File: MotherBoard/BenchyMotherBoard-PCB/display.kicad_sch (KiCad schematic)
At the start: 13 parts

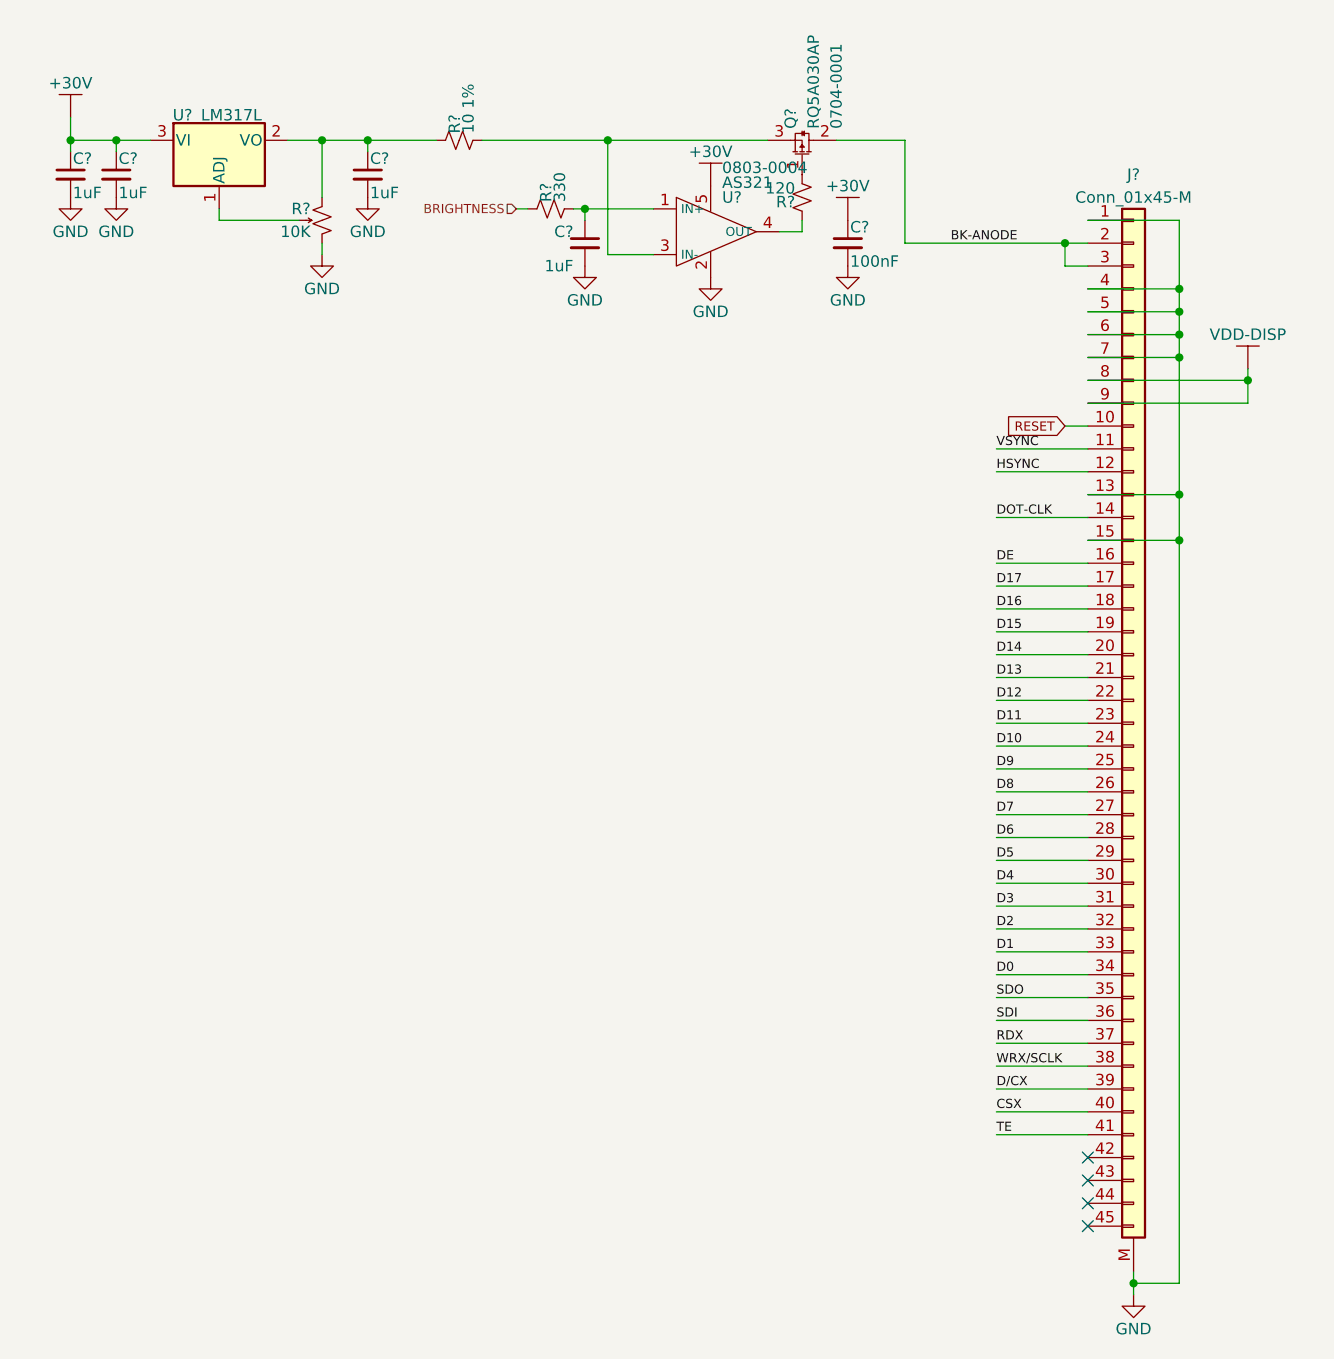
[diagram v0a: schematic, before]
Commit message: Initial schematic lock
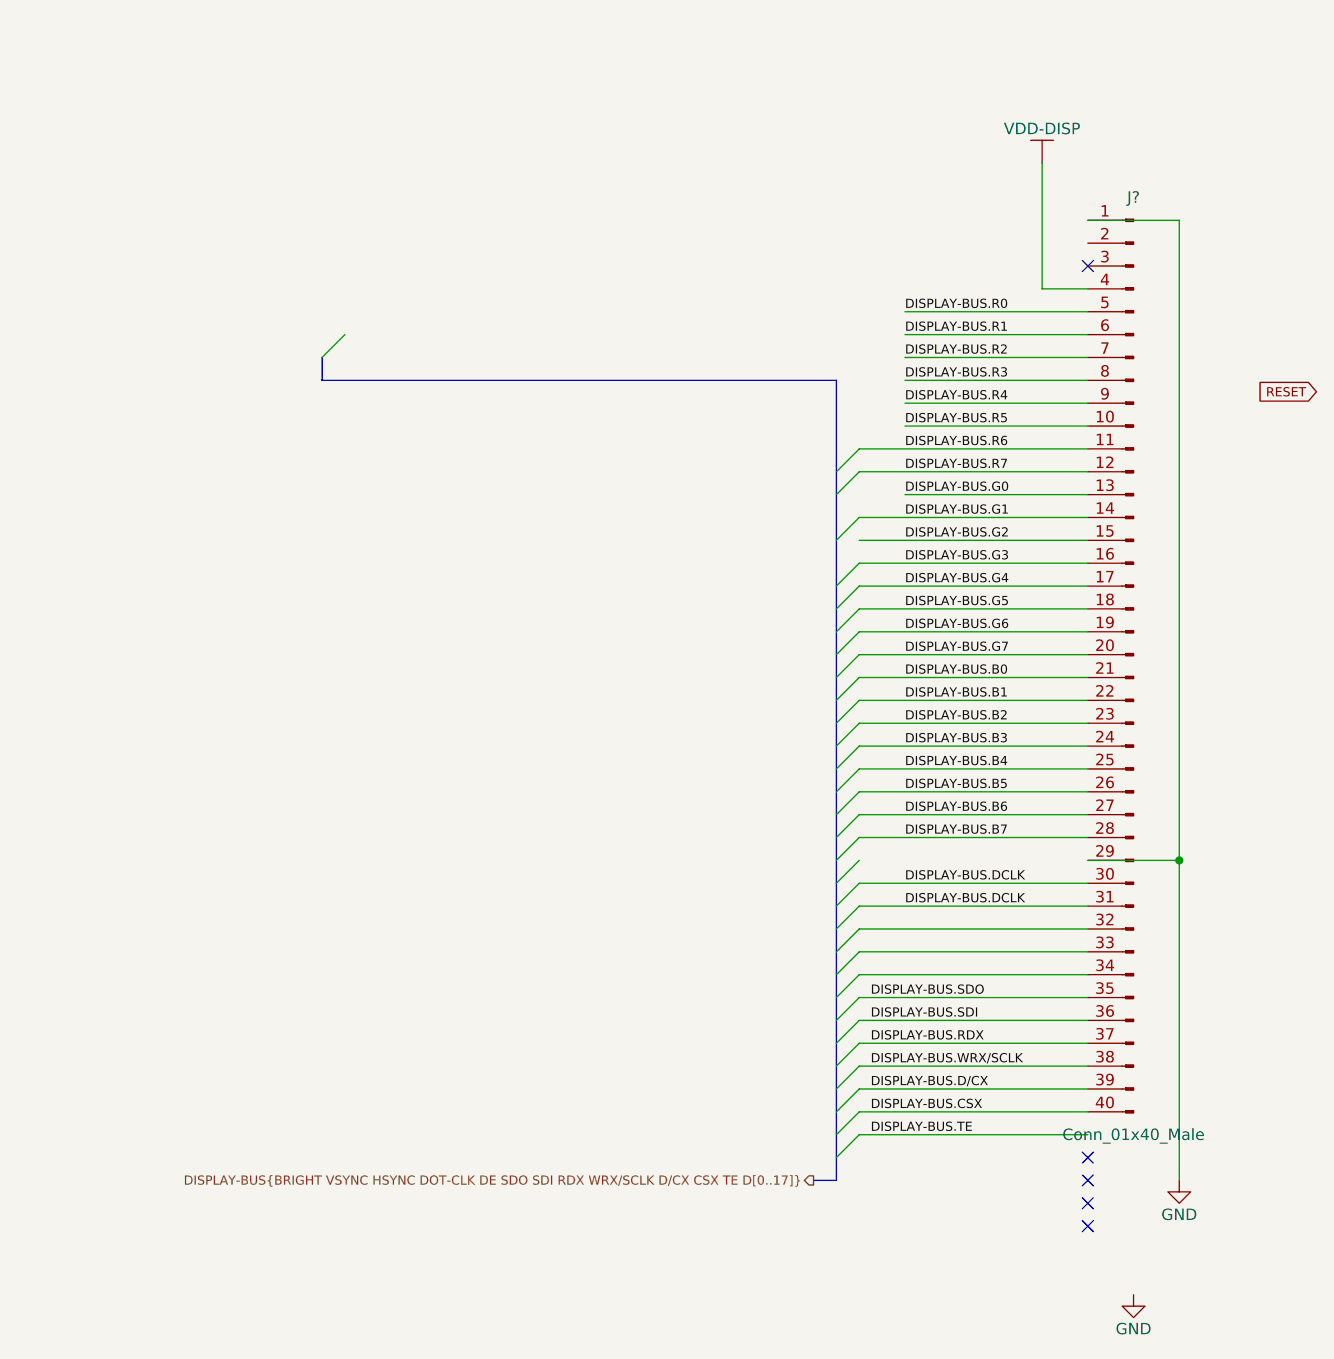
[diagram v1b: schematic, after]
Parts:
- removed C?: 1uF, symbol Device:C_Small
- removed C?: 1uF, Capacitor_SMD:C_0805_2012Metric, symbol Device:C_Small
- removed C? (x2): 1uF, Capacitor_SMD:C_1210_3225Metric, symbol Device:C_Small
- removed C?: 100nF, Capacitor_SMD:C_0805_2012Metric, symbol Device:C_Small
- removed J?: Conn_01x45-M, Daxxn_Connectors:046841045100846+, symbol Daxxn_Connectors:Conn_01x45-M
- removed Q?: RQ5A030AP, Package_TO_SOT_SMD:SOT-23, symbol Daxxn_Transistors:RQ5A030AP
- removed R?: 120, Resistor_SMD:R_0805_2012Metric, symbol Device:R_Small_US
- removed R?: 10K, symbol Daxxn_Other:R_Pot_Small_US
- removed R?: 330, Resistor_SMD:R_0805_2012Metric, symbol Device:R_Small_US
- removed R?: 10 1%, Resistor_SMD:R_0805_2012Metric, symbol Device:R_Small_US
- removed U?: AS321, Package_TO_SOT_SMD:SOT-23-5, symbol Daxxn_OPAMP:AS321
- removed U?: LM317L, Package_TO_SOT_SMD:SOT-89-3, symbol Regulator_Linear:LM317L_SOT-89
- added J?: Conn_01x40_Male, symbol Connector:Conn_01x40_Male
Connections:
- net GND: now also J?.1 (Pin_1), J?.29 (Pin_29)
- net VDD-DISP: now also J?.4 (Pin_4)
- new net DISPLAY-BUS.B0: J?.21 (Pin_21)
- new net DISPLAY-BUS.B1: J?.22 (Pin_22)
- new net DISPLAY-BUS.B2: J?.23 (Pin_23)
- new net DISPLAY-BUS.B3: J?.24 (Pin_24)
- new net DISPLAY-BUS.B4: J?.25 (Pin_25)
- new net DISPLAY-BUS.B5: J?.26 (Pin_26)
- new net DISPLAY-BUS.B6: J?.27 (Pin_27)
- new net DISPLAY-BUS.B7: J?.28 (Pin_28)
- new net DISPLAY-BUS.CSX: J?.40 (Pin_40)
- new net DISPLAY-BUS.DCLK: J?.30 (Pin_30), J?.31 (Pin_31)
- new net DISPLAY-BUS.D/CX: J?.39 (Pin_39)
- new net DISPLAY-BUS.G0: J?.13 (Pin_13)
- new net DISPLAY-BUS.G1: J?.14 (Pin_14)
- new net DISPLAY-BUS.G2: J?.15 (Pin_15)
- new net DISPLAY-BUS.G3: J?.16 (Pin_16)
- new net DISPLAY-BUS.G4: J?.17 (Pin_17)
- new net DISPLAY-BUS.G5: J?.18 (Pin_18)
- new net DISPLAY-BUS.G6: J?.19 (Pin_19)
- new net DISPLAY-BUS.G7: J?.20 (Pin_20)
- new net DISPLAY-BUS.R0: J?.5 (Pin_5)
- new net DISPLAY-BUS.R1: J?.6 (Pin_6)
- new net DISPLAY-BUS.R2: J?.7 (Pin_7)
- new net DISPLAY-BUS.R3: J?.8 (Pin_8)
- new net DISPLAY-BUS.R4: J?.9 (Pin_9)
- new net DISPLAY-BUS.R5: J?.10 (Pin_10)
- new net DISPLAY-BUS.R6: J?.11 (Pin_11)
- new net DISPLAY-BUS.R7: J?.12 (Pin_12)
- new net DISPLAY-BUS.RDX: J?.37 (Pin_37)
- new net DISPLAY-BUS.SDI: J?.36 (Pin_36)
- new net DISPLAY-BUS.SDO: J?.35 (Pin_35)
- new net DISPLAY-BUS.WRX/SCLK: J?.38 (Pin_38)
- no-connect marks 4 -> 5
